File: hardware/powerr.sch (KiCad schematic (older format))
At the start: 33 parts, among them P24 CONN_01X02, U26 OKR_T3, U41 OKR_T3, U45 OKR_T3, U50 LT3010, X3 RKZ1215D

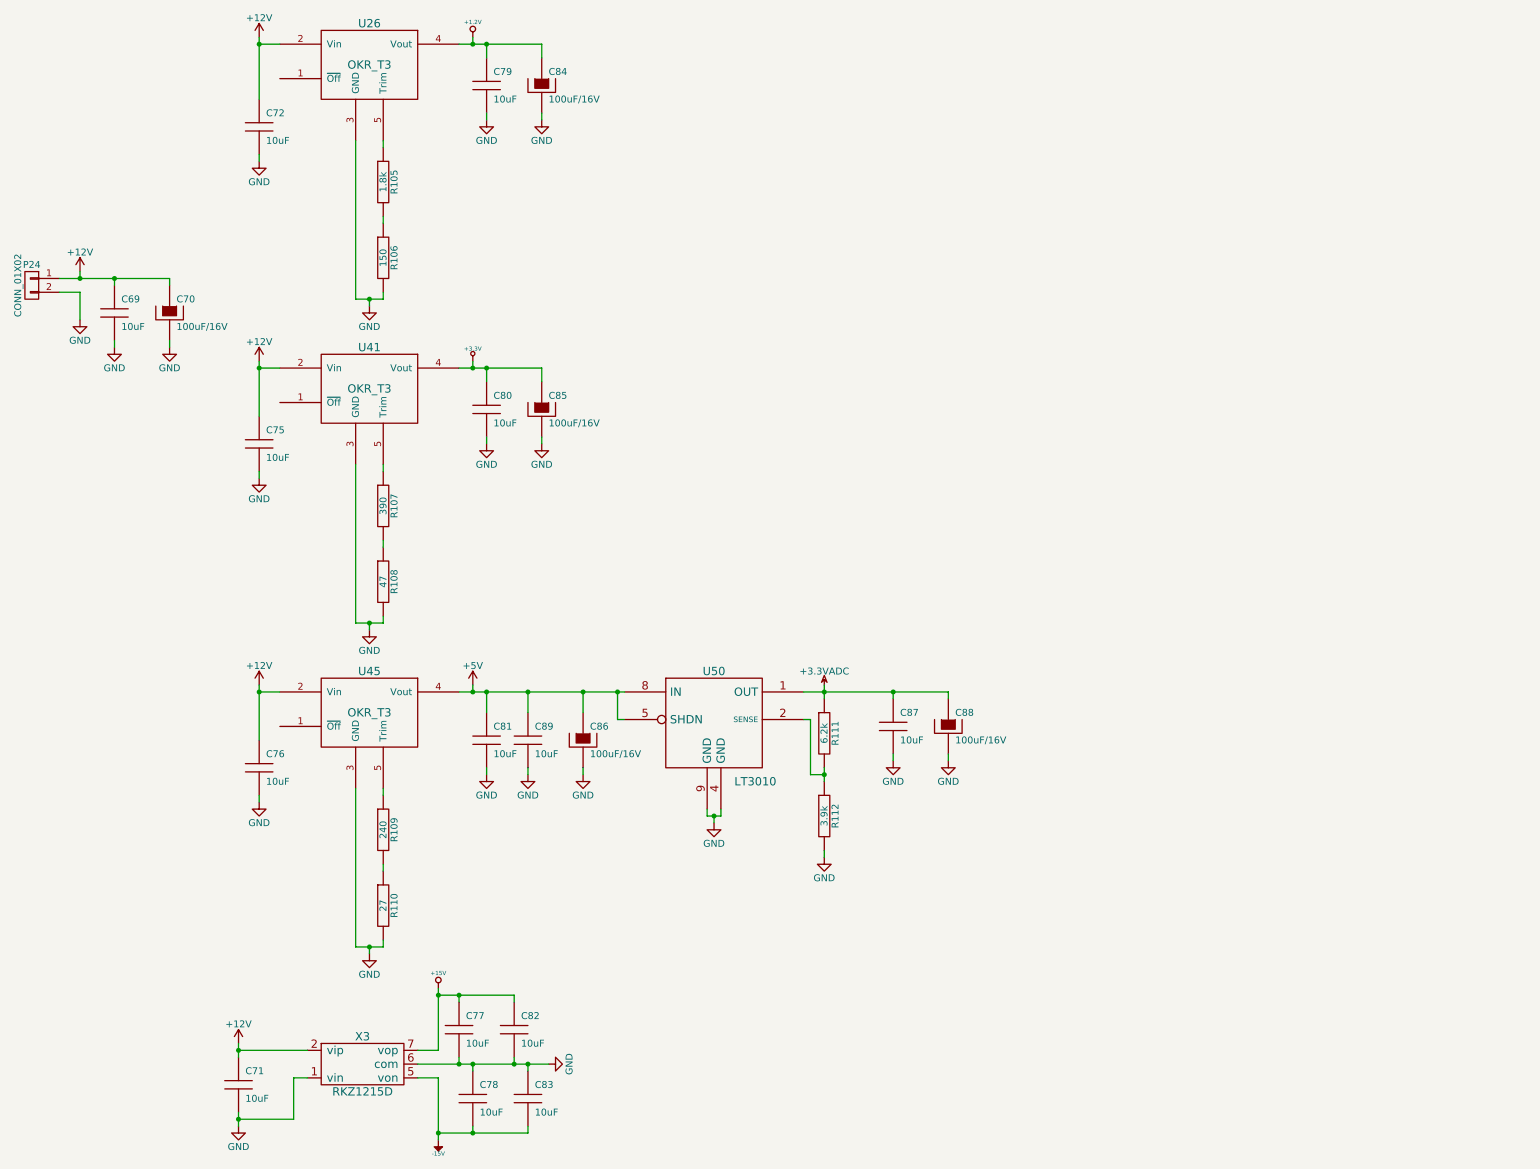
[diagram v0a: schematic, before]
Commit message: Backup
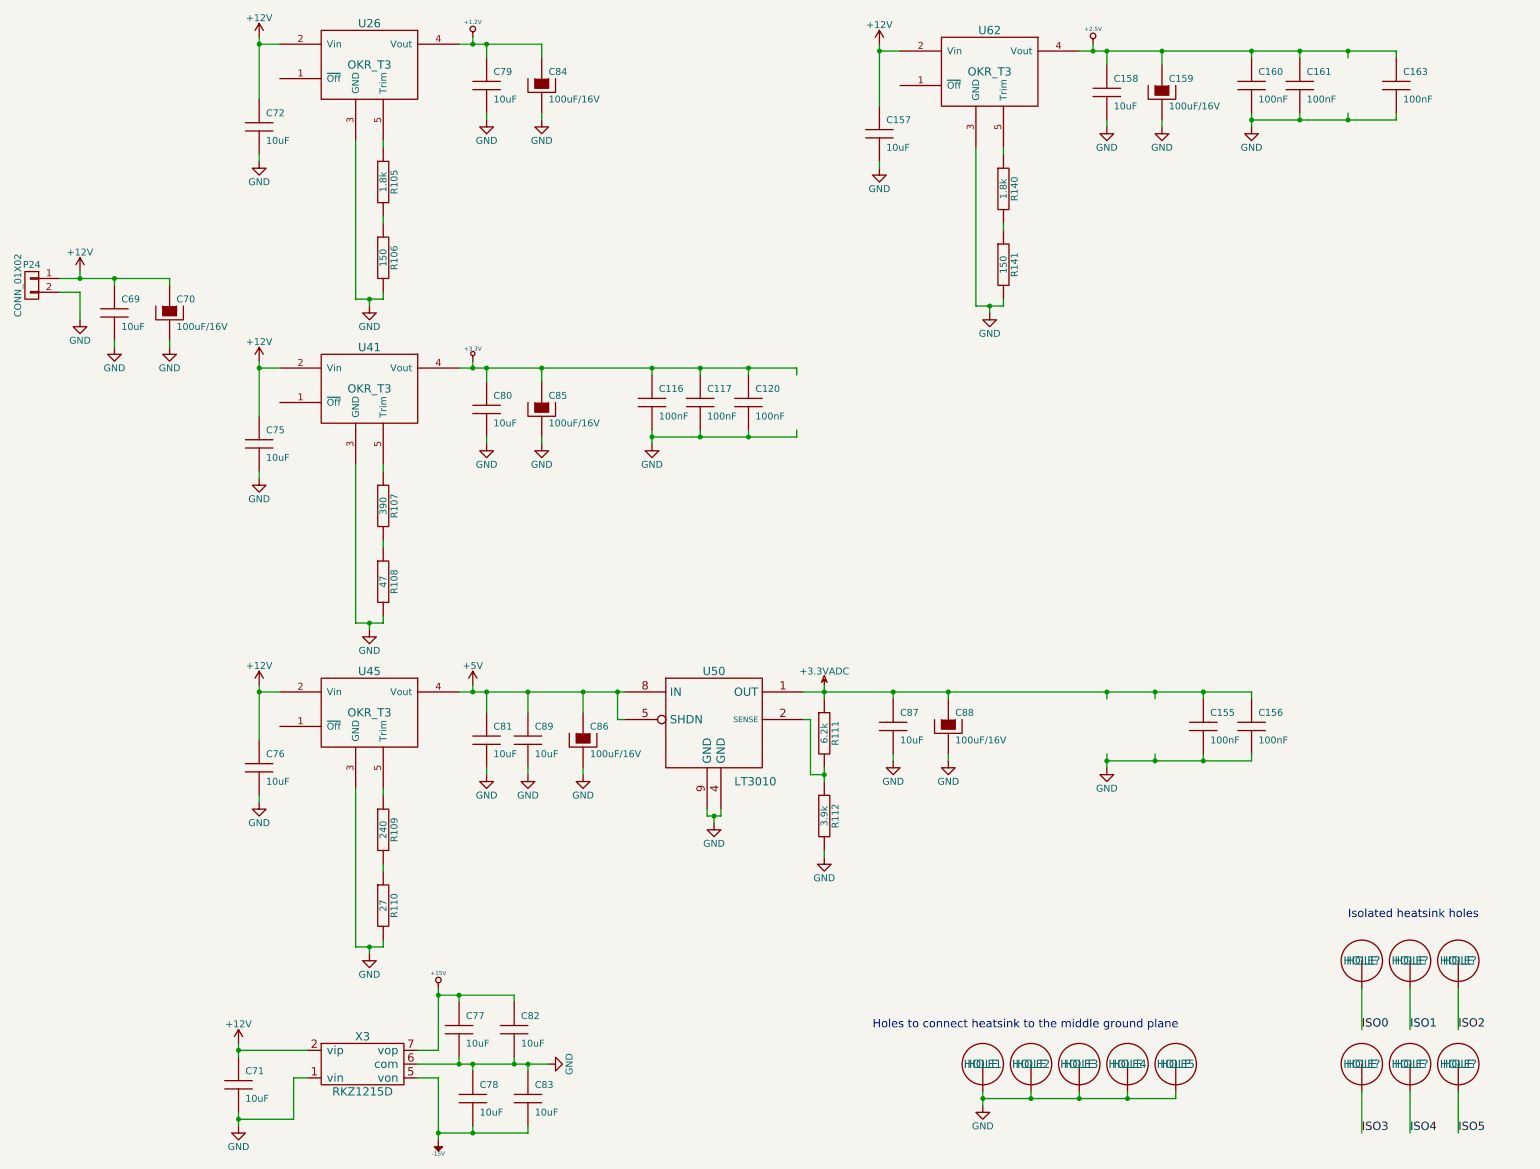
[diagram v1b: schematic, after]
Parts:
- added C116, C117, C120, C155, C156, C160, C161, C163: 100nF, 00_Passives:C0603, symbol C
- added C157, C158: 10uF, 00_Passives:C1210, symbol C
- added C159: 100uF/16V, Capacitors_SMD:c_elec_6.3x5.3, symbol CAPAPOL
- added HOLE1, HOLE2, HOLE3, HOLE4, HOLE5, HOLE? (x6): HOLE, 00_Local:hole_3mm, symbol HOLE
- added R140: 1.8k, 00_Passives:R0603, symbol R
- added R141: 150, 00_Passives:R0603, symbol R
- added U62: OKR_T3, 00_Passives:okr_t3, symbol OKR_T3
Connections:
- net labels added: +2.5V, ISO0, ISO1, ISO2, ISO3, ISO4, ISO5
- wire segments 93 -> 147
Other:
- note added: "Holes to connect heatsink to the middle ground plane"
- note added: "Isolated heatsink holes"

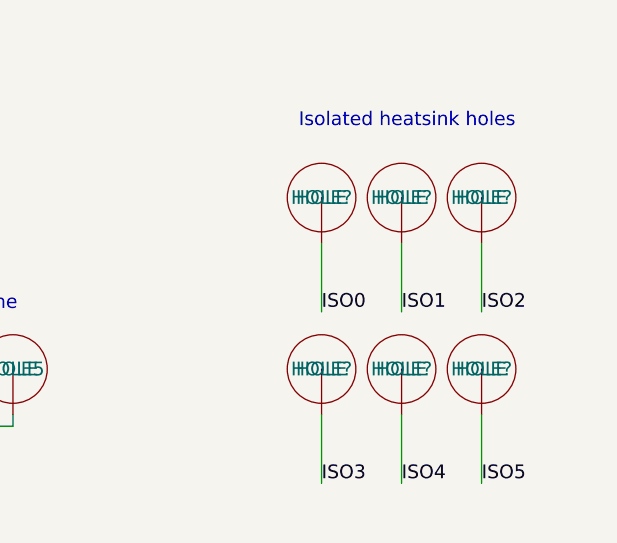
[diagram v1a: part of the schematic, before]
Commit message: First small drive hardware.
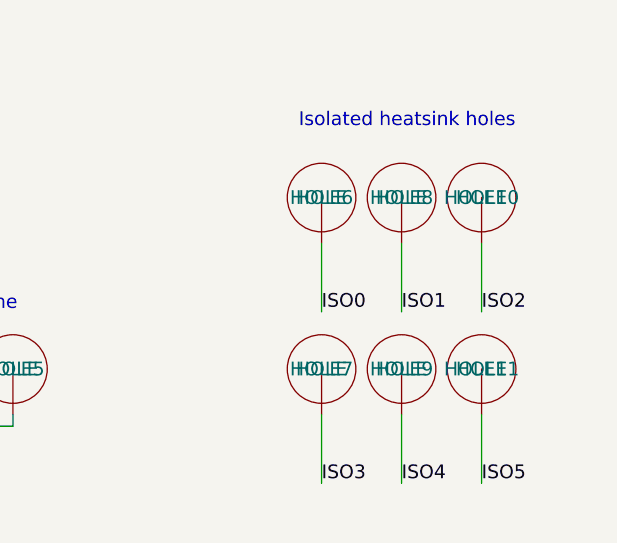
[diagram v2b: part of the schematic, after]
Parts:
- gave numbers to parts that had none: 6
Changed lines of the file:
@@
 Connection ~ 9900 8600
 $Comp
-L HOLE HOLE?
+L HOLE HOLE6
 U 1 1 56F34D98
 P 11600 7600
-F 0 "HOLE?" H 11600 7600 60  0000 C CNN
+F 0 "HOLE6" H 11600 7600 60  0000 C CNN
 F 1 "HOLE" H 11600 7600 60  0000 C CNN
 F 2 "00_Local:hole_3mm" H 11600 7600 60  0001 C CNN
@@
 Isolated heatsink holes
 $Comp
-L HOLE HOLE?
+L HOLE HOLE8
 U 1 1 56F350D1
 P 11950 7600
-F 0 "HOLE?" H 11950 7600 60  0000 C CNN
+F 0 "HOLE8" H 11950 7600 60  0000 C CNN
 F 1 "HOLE" H 11950 7600 60  0000 C CNN
 F 2 "00_Local:hole_3mm" H 11950 7600 60  0001 C CNN
@@
 	11950 7800 11950 8100
 $Comp
-L HOLE HOLE?
+L HOLE HOLE10
 U 1 1 56F3511E
 P 12300 7600
-F 0 "HOLE?" H 12300 7600 60  0000 C CNN
+F 0 "HOLE10" H 12300 7600 60  0000 C CNN
 F 1 "HOLE" H 12300 7600 60  0000 C CNN
 F 2 "00_Local:hole_3mm" H 12300 7600 60  0001 C CNN
@@
 	12300 7800 12300 8100
 $Comp
-L HOLE HOLE?
+L HOLE HOLE7
 U 1 1 56F351DA
 P 11600 8350
-F 0 "HOLE?" H 11600 8350 60  0000 C CNN
+F 0 "HOLE7" H 11600 8350 60  0000 C CNN
 F 1 "HOLE" H 11600 8350 60  0000 C CNN
 F 2 "00_Local:hole_3mm" H 11600 8350 60  0001 C CNN
@@
 	11600 8550 11600 8850
 $Comp
-L HOLE HOLE?
+L HOLE HOLE9
 U 1 1 56F351E1
 P 11950 8350
-F 0 "HOLE?" H 11950 8350 60  0000 C CNN
+F 0 "HOLE9" H 11950 8350 60  0000 C CNN
 F 1 "HOLE" H 11950 8350 60  0000 C CNN
 F 2 "00_Local:hole_3mm" H 11950 8350 60  0001 C CNN
@@
 	11950 8550 11950 8850
 $Comp
-L HOLE HOLE?
+L HOLE HOLE11
 U 1 1 56F351E8
 P 12300 8350
-F 0 "HOLE?" H 12300 8350 60  0000 C CNN
+F 0 "HOLE11" H 12300 8350 60  0000 C CNN
 F 1 "HOLE" H 12300 8350 60  0000 C CNN
 F 2 "00_Local:hole_3mm" H 12300 8350 60  0001 C CNN
